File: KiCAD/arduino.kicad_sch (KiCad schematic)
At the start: 2 parts, among them U1 Si5351A_Breakout, U2 Metro_ESP32S3

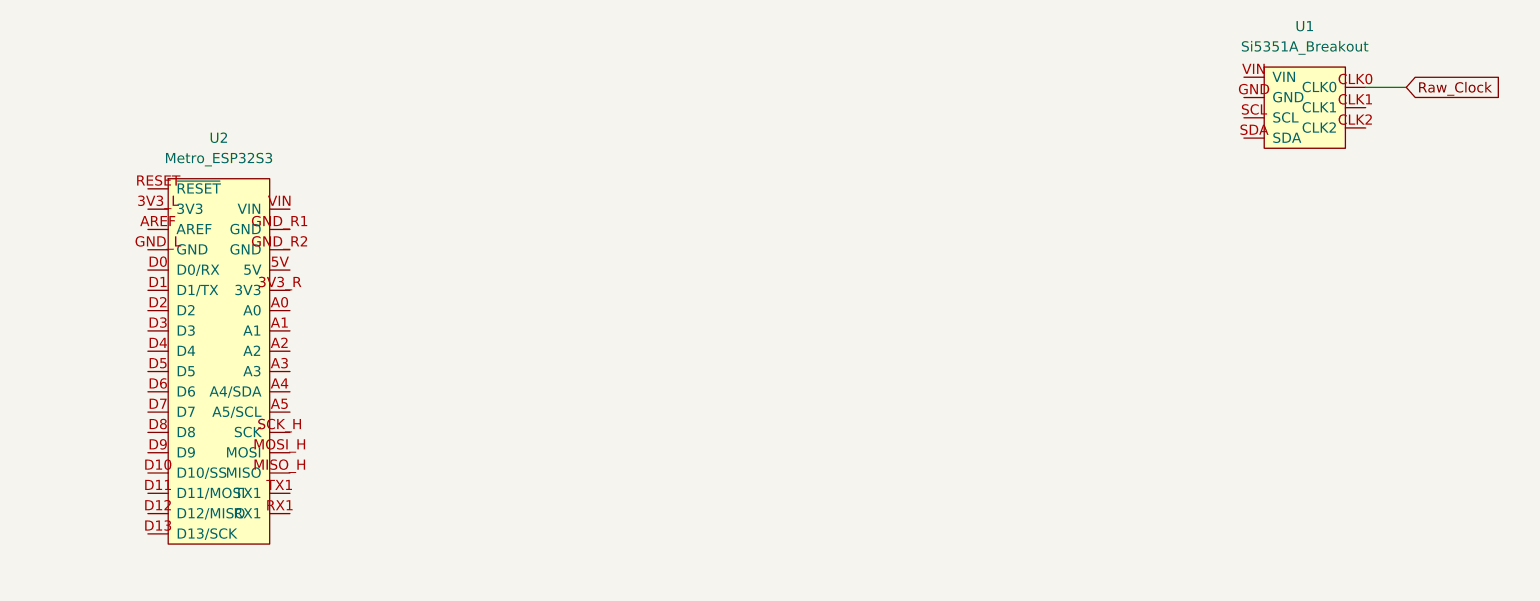
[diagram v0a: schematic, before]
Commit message: Work in Progress
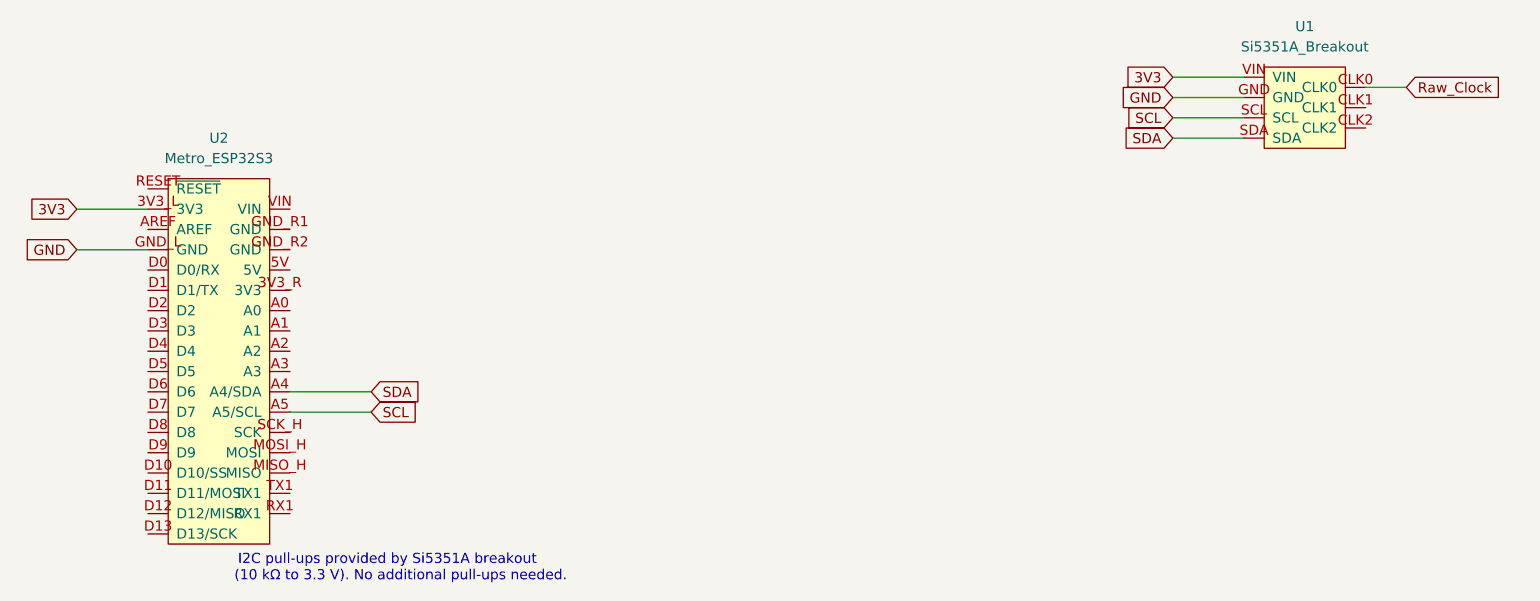
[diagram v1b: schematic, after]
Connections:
- net 3V3: now reaches U2.3V3_L (3V3)
- net 3V3: now also U1.VIN
- net SDA: now reaches U2.A4 (A4/SDA)
- net SDA: now also U1.SDA
- net SCL: now reaches U2.A5 (A5/SCL)
- net SCL: now also U1.SCL
- net GND: now reaches U2.GND_L (GND)
- net GND: now also U1.GND
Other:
- note added: "I2C pull-ups provided by Si5351A breakout (10 kΩ to 3.3 V). No additional pull-ups needed."
